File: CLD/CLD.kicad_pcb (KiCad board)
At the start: 2 copper layers, 56.2 x 33 mm, 26 parts, among them J1 Conn_01x02, J2 Conn_01x02, J3 Conn_01x02, J4 Conn_01x02, J5 Conn_02x05_Counter_Clockwise, Q1 BSC072N08NS5, U1 STM32F103CBUx, U2 FAN3111E, U3 INA180A1, U4 MCP2551-I-SN

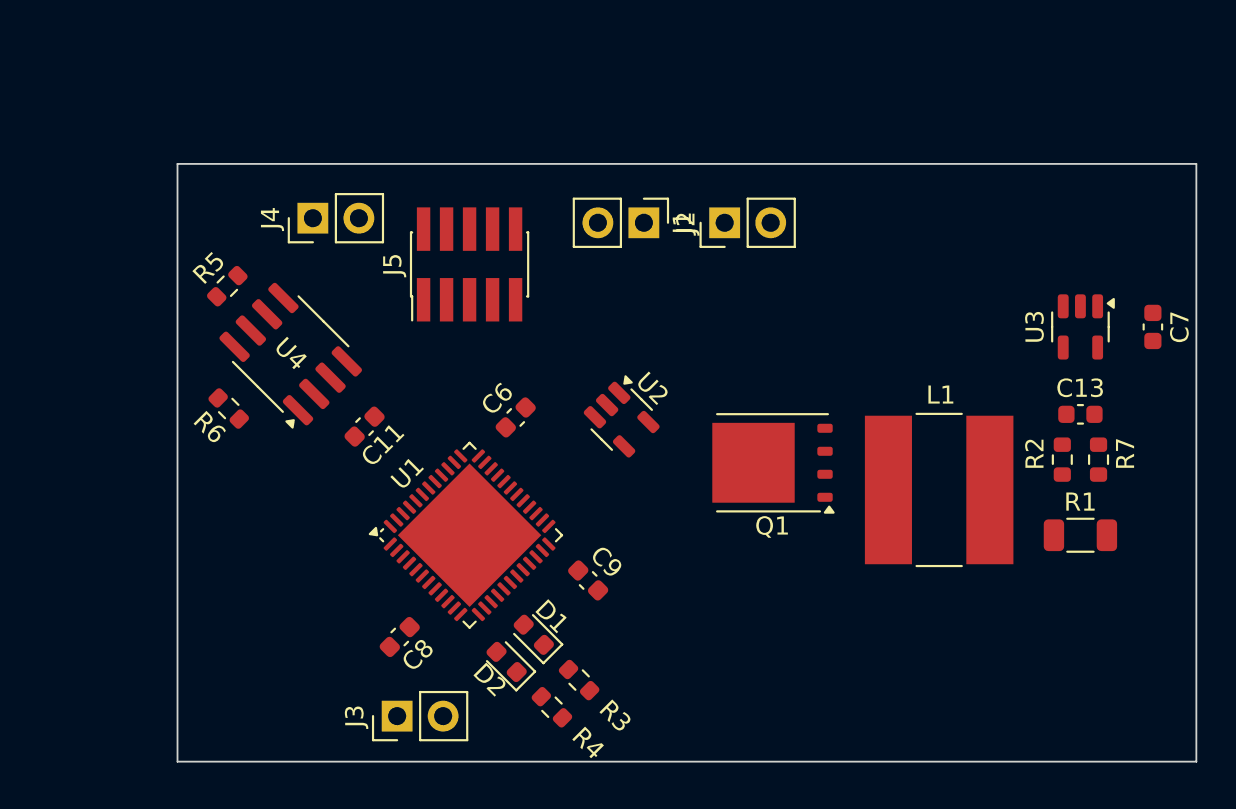
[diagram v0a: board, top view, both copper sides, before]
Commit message: howdy
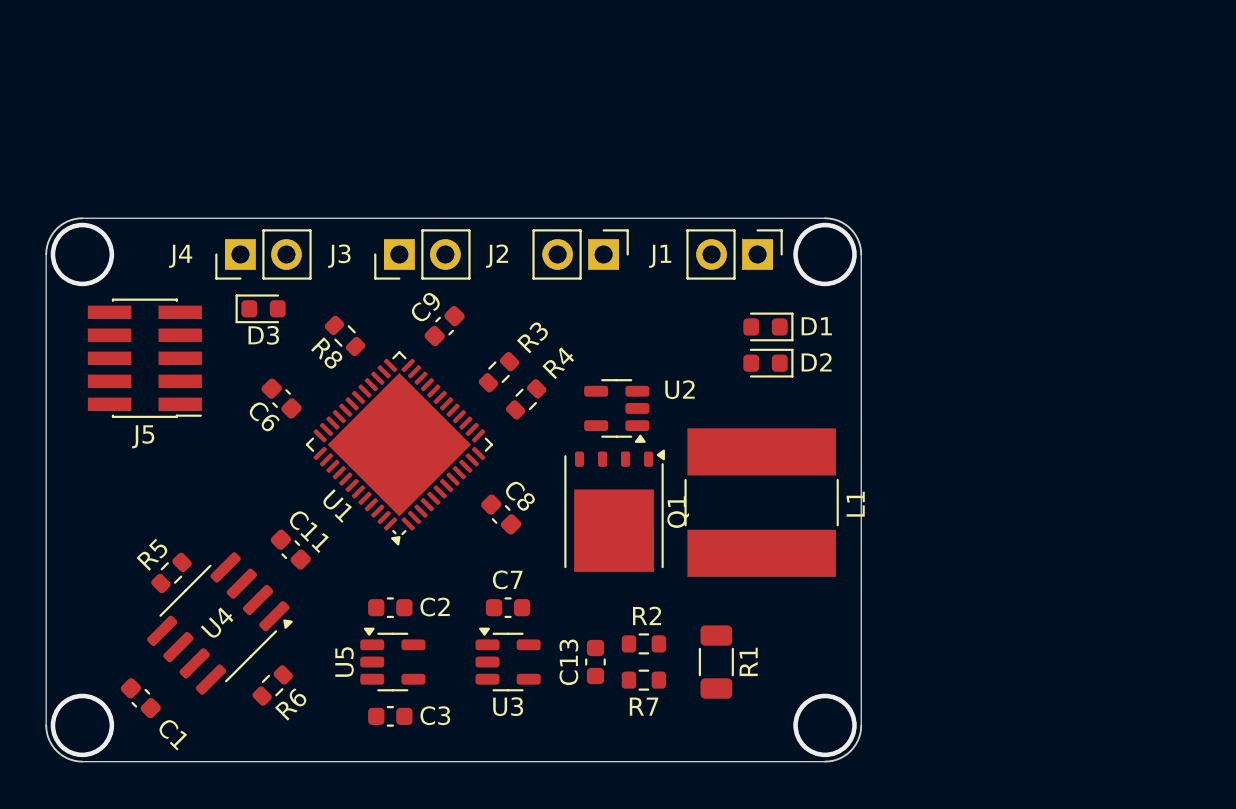
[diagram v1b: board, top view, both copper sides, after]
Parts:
- added C1: 100n, Capacitor_SMD:C_0603_1608Metric, F.Cu at (78.7, 79.0)
- added C2: 100n, Capacitor_SMD:C_0603_1608Metric, F.Cu at (92.5, 74.0)
- added C3: 100n, Capacitor_SMD:C_0603_1608Metric, F.Cu at (92.5, 80.0)
- added D3: LED, Diode_SMD:D_0603_1608Metric, F.Cu at (85.5, 57.5)
- added R8: 50r, Resistor_SMD:R_0603_1608Metric, F.Cu at (90.0, 59.0)
- added U5: AP2112K-3.3, Package_TO_SOT_SMD:SOT-23-5, F.Cu at (92.6, 77.0)
- R3, R4: value R -> 50r
- moved C7 38.8 mm to (99.0, 74.0), turned to 180 degrees
- moved U3 36.6 mm to (99.0, 77.0), turned to 0 degrees
- moved C13 30.1 mm to (103.8, 77.0), turned to 90 degrees
- moved R7 27.9 mm to (106.5, 78.0), turned to 180 degrees
- moved J3 25.5 mm to (93.0, 54.5)
- moved R2 25.2 mm to (106.5, 76.0), turned to 180 degrees
- moved D2 21.8 mm to (113.2, 60.5), turned to 180 degrees
- moved R1 21.3 mm to (110.5, 77.0), turned to -90 degrees
- moved D1 21.3 mm to (113.2, 58.5), turned to 180 degrees
- moved J5 18.7 mm to (79.0, 60.2), turned to 180 degrees
- moved R3 17.6 mm to (98.5, 61.0), turned to 45 degrees
- moved R4 17.1 mm to (100.0, 62.5), turned to 45 degrees
- moved R5 16.1 mm to (80.4, 72.1)
- moved C9 16.1 mm to (95.5, 58.5), turned to 45 degrees
- moved R6 15.5 mm to (86.0, 78.3), turned to 45 degrees
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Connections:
- D1 pad 1: Net-(D1-K) -> GND
- D2 pad 1: Net-(D2-K) -> GND
- R3 pad 1: Net-(D1-K) -> Net-(U1-PA4)
- R3 pad 2: GND -> Net-(D1-A)
- R4 pad 1: Net-(D2-K) -> Net-(U1-PA3)
- R4 pad 2: GND -> Net-(D2-A)
- U1 pad 13: Net-(D2-A) -> Net-(U1-PA3)
- U1 pad 14: Net-(D1-A) -> Net-(U1-PA4)
- U1 pad 26: unconnected-(U1-PB13-Pad26) -> Net-(U1-PB13)
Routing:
- net GND: vias 0 -> 4
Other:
- board size 56.2 x 33 mm -> 45 x 30 mm

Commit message: PCB routed
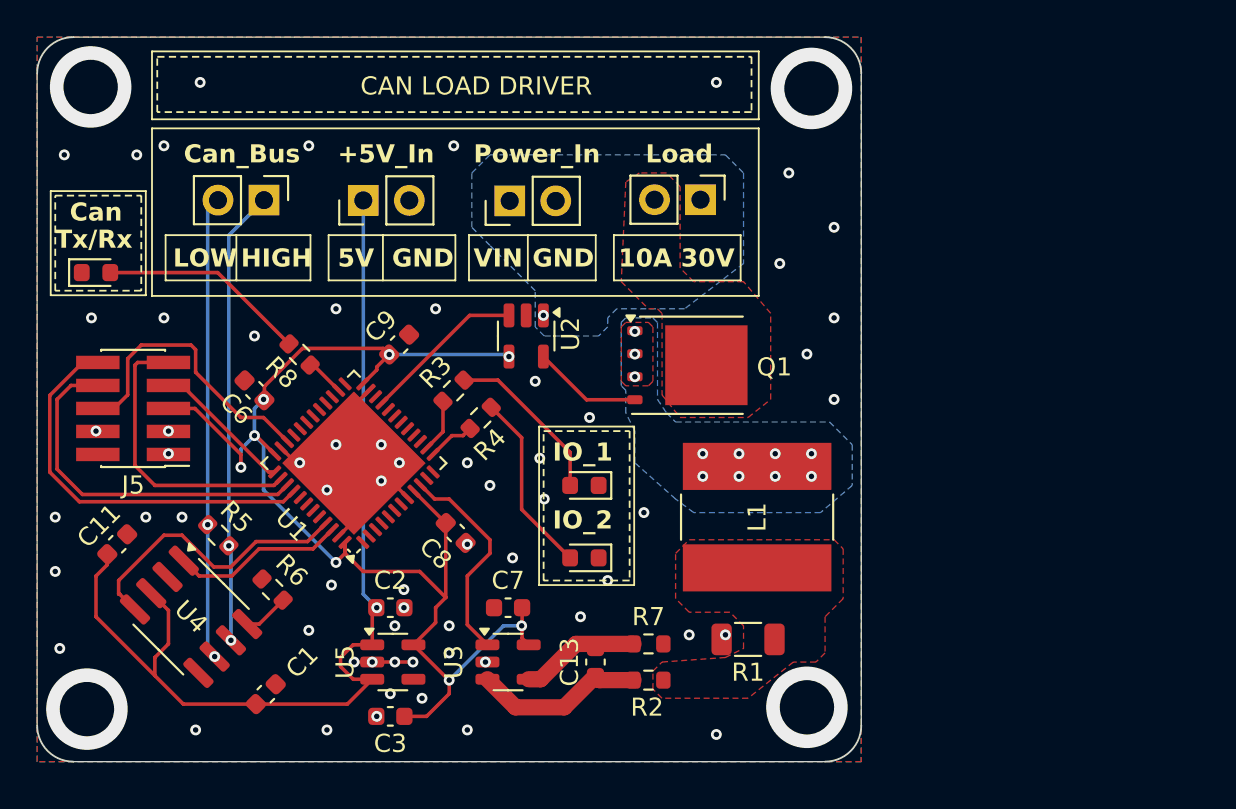
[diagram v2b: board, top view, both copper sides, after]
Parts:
- moved D2 14.7 mm to (103.2, 71.2)
- moved D1 13.3 mm to (103.2, 67.2)
- moved C11 9.59 mm to (77.4, 70.5), turned to 45 degrees
- moved D3 9.46 mm to (76.2, 55.5)
- moved Q1 9.04 mm to (108.9, 60.6), turned to 0 degrees
- moved C1 6.90 mm to (85.6, 78.8), turned to 45 degrees
- moved U2 6.40 mm to (100.0, 59.0), turned to -90 degrees
- moved J2 5.97 mm to (99.1, 51.5), turned to 90 degrees
- moved R6 5.30 mm to (86.0, 73.0), turned to 135 degrees
- moved J1 4.37 mm to (109.6, 51.5)
- moved J3 3.59 mm to (91.0, 51.5)
- moved R5 3.32 mm to (83.0, 70.0), turned to 135 degrees
- moved J4 3.27 mm to (85.5, 51.5), turned to -90 degrees
- moved J5 2.85 mm to (78.3, 63.0)
- moved C9 2.71 mm to (93.0, 59.5)
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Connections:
- U1 pad 15: /Mos_EN -> unconnected-(U1-PA5-Pad15)
- U1 pad 21: unconnected-(U1-PB10-Pad21) -> /Mos_EN
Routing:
- net +3.3V: track 0.00 -> 70.4 mm, vias 0 -> 8
- net +5V: track 0.00 -> 56.4 mm, vias 0 -> 1
- net /Can_L: track 0.00 -> 25.6 mm, vias 0 -> 2
- net /Can_H: track 0.00 -> 25.2 mm, vias 0 -> 2
- net /JTAG_RST: track 0.00 -> 22.0 mm
- net GND: track 0.00 -> 20.1 mm, vias 4 -> 68
- net /JTAG_D0: track 0.00 -> 19.6 mm
- net /JTAG_SWDIO: track 0.00 -> 16.3 mm
- net /Can_Rx: track 0.00 -> 16.2 mm
- net /JTAG_D1: track 0.00 -> 15.8 mm
- net /Current: track 0.00 -> 11.9 mm
- net Net-(D3-A): track 0.00 -> 11.5 mm
- net Net-(D2-A): track 0.00 -> 10.1 mm
- net /Can_Tx: track 0.00 -> 9.61 mm
- net Net-(U3-+): track 0.00 -> 9.51 mm
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- added copper zone on B.Cu, net GND
- added copper zone on F.Cu, net GND
- added copper zone on F.Cu, net Net-(J1-Pin_2)
- added copper zone on B.Cu, net Net-(L1-Pad1)
- added copper zone on F.Cu, net Net-(L1-Pad1)
- added copper zone on F.Cu, net Net-(L1-Pad2)
- added copper zone on B.Cu, net VDD
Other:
- board size 45 x 30 mm -> 45.5 x 40 mm
- board text added: "+5V_In"
- board text added: "10A 30V"
- board text added: "5V"
- board text added: "CAN LOAD DRIVER"
- board text added: "Can"
- board text added: "Can_Bus"
- board text added: "GND"
- board text added: "HIGH"
- board text added: "IO_1"
- board text added: "IO_2"
- board text added: "LOW"
- board text added: "Load"
- board text added: "Power_In"
- board text added: "Tx/Rx"
- board text added: "VIN"
